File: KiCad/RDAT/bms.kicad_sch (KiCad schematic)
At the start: 37 parts, among them Q1 NMOS, Q2 NMOS, U3 BQ7791500PWT, U4 BQ34Z100PWR-R2

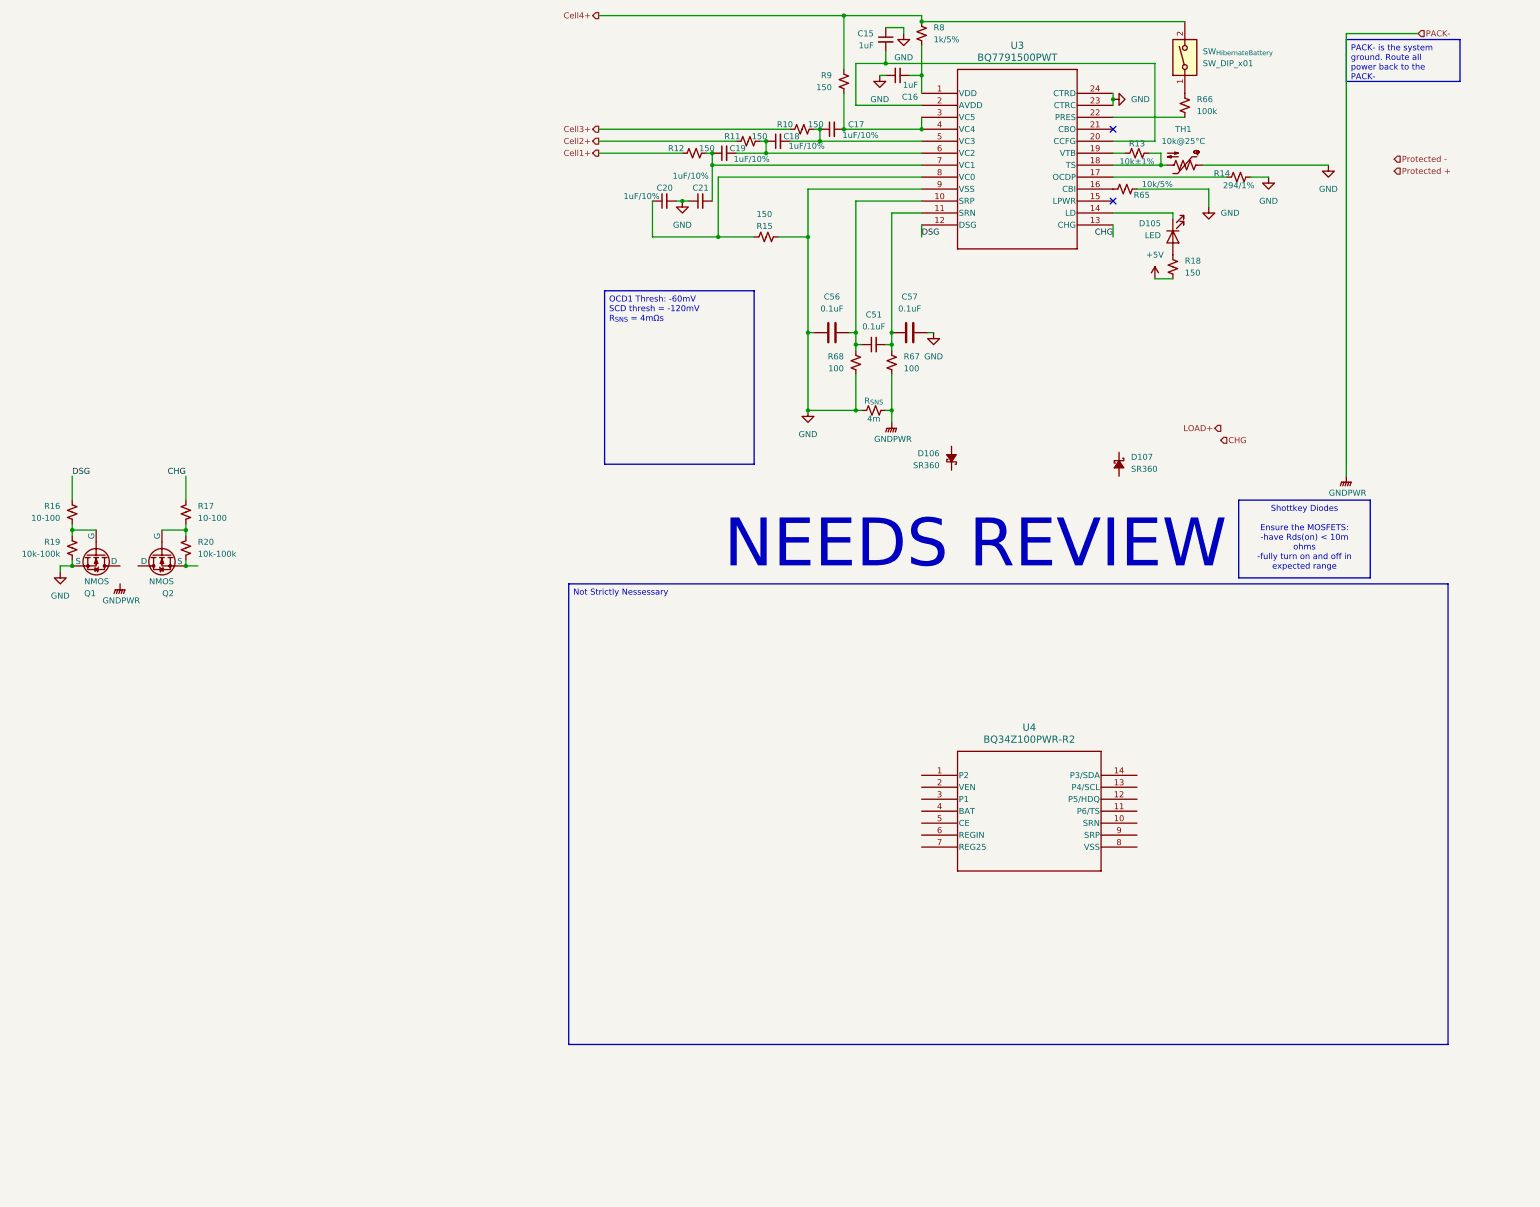
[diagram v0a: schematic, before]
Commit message: 2x checked all schematics
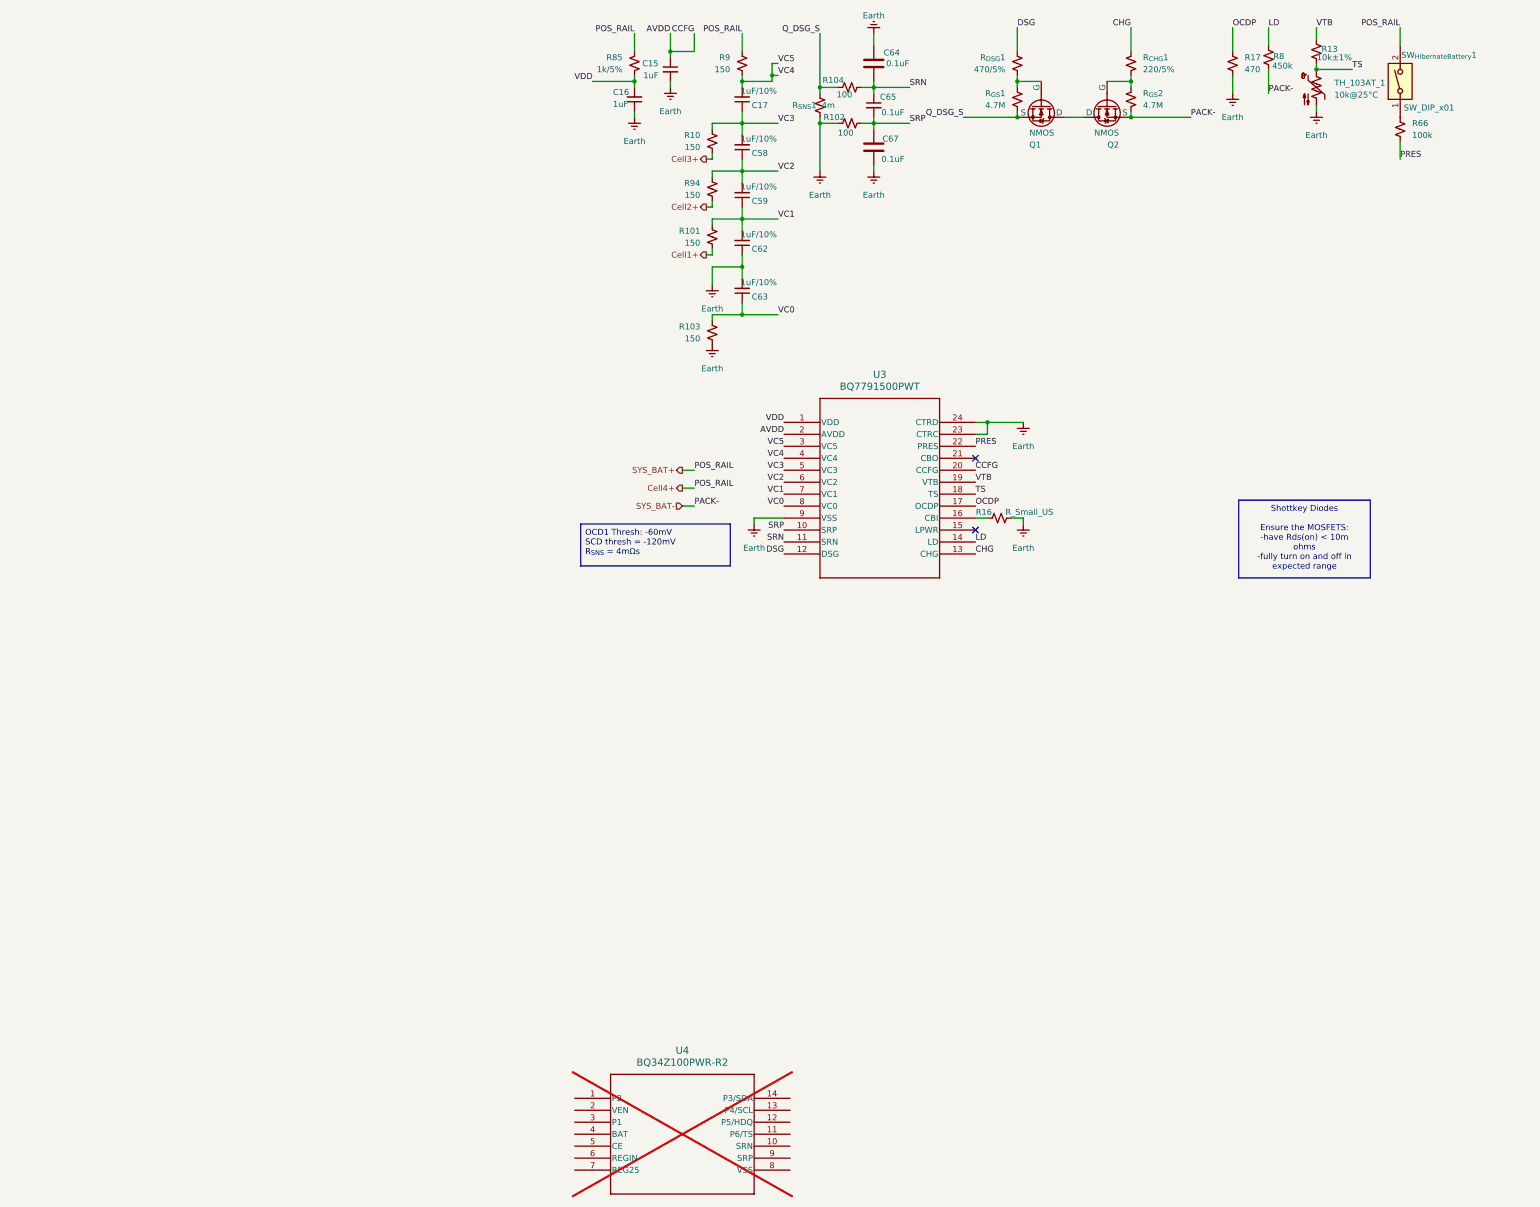
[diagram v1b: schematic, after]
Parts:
- removed C18, C19, C20, C21: 1uF/10%, symbol Device:C_Small
- removed C51: 0.1uF, symbol Device:C_Small
- removed C56, C57: 0.1uF, symbol Device:C
- removed D105: LED, symbol Device:LED
- removed D106, D107: SR360, symbol Device:D_Schottky_Small_Filled
- removed R11, R12, R15, R18: 150, symbol Device:R_Small_US
- removed R14: 294/1%, symbol Device:R_Small_US
- removed R65: 10k/5%, symbol Device:R_Small_US
- removed R67, R68: 100, symbol Device:R_Small_US
- removed R_{SNS}: 4m, symbol Device:R_Small_US
- added C58, C59, C62, C63: 1uF/10%, symbol Device:C_Small
- added C64, C67: 0.1uF, symbol Device:C
- added C65: 0.1uF, symbol Device:C_Small
- added R101, R103, R94: 150, symbol Device:R_Small_US
- added R102, R104: 100, symbol Device:R_Small_US
- added R16: R_Small_US, symbol Device:R_Small_US
- added R17: 470, symbol Device:R_Small_US
- added R85: 1k/5%, symbol Device:R_Small_US
- added R_{SNS}1: 4m, symbol Device:R_Small_US
- R8: value 1k/5% -> 450k
- R_{CHG}1: renamed from R17; value 10-100 -> 220/5%
- R_{DSG}1: renamed from R16; value 10-100 -> 470/5%
- R_{GS}1: renamed from R19; value 10k-100k -> 4.7M
- R_{GS}2: renamed from R20; value 10k-100k -> 4.7M
- U4: now not fitted
- renumbered SW_{HibernateBattery} to SW_{HibernateBattery}1, TH1 to TH_103AT_1
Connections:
- net Cell1+: now also R101.2
- net Cell2+: now also R94.2
- net Cell3+: now also R10.2; no longer R10.1
- net Cell4+: now also R85.1; no longer R8.1
- net SRP: now reaches U3.10 (SRP)
- net SRP: now also C65.2, C67.1, R102.2
- net SRN: now reaches U3.11 (SRN)
- net SRN: now also C64.2, C65.1, R104.2
- net at Q2.1 (D): now also Q1.1 (D)
- net SYS_BAT-: now reaches Q2.3 (S), R_{GS}2.2
- net SYS_BAT-: now also R8.2
- net TS: now reaches R13.1
- net TS: now also TH_103AT_1.1, U3.18 (TS); no longer U3.19 (VTB)
- net VC0: now reaches U3.8 (VC0)
- net VC0: now also C63.1, R103.1
- net VC2: now reaches U3.6 (VC2)
- net VC2: now also C58.1, C59.2, R94.1
- net VC1: now reaches U3.7 (VC1)
- net VC1: now also C59.1, C62.2, R101.1
- net VC3: now reaches C17.1, U3.5 (VC3)
- net VC3: now also R10.1, C58.2; no longer R10.2
- net VDD: now reaches C16.2, U3.1 (VDD)
- net VDD: now also R85.2; no longer R8.2
- net PRES: now reaches R66.2, U3.22 (PRES)
- net at U3.16 (CBI): now also R16.1
- net VC4: now reaches C17.2, R9.2, U3.3 (VC5), U3.4 (VC4)
- net OCDP: now reaches U3.17 (OCDP)
- net OCDP: now also R17.1
- net LD: now reaches U3.14 (LD)
- net LD: now also R8.1
- net AVDD: now reaches U3.2 (AVDD), U3.20 (CCFG)
- net AVDD: now also C15.1; no longer C15.2
- net GND renamed Earth
- net Earth: now also C15.2, TH_103AT_1.2, C62.1, C63.2, C64.1, C67.2, R102.1, R103.2, R16.2, R17.2, R_{SNS}1.1; no longer C15.1, Q1.3 (S), R_{GS}1.2, TH_103AT_1.1
- new net Q_DSG_S: Q1.3 (S), R104.1, R_{GS}1.2, R_{SNS}1.2
- new net VTB: R13.2, U3.19 (VTB)
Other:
- note removed: "NEEDS REVIEW"
- moved on the sheet: C15, C16, C17, Q1, Q2, R13, R66, R9, R_{CHG}1, R_{DSG}1, R_{GS}1, R_{GS}2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
